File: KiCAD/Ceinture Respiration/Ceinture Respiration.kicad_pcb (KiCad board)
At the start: 4 copper layers, 45 x 82.8 mm, 39 parts, among them J1 Conn_01x10_Pin, J10 BUZZER, J11 Conn_01x02, J2 Conn_01x10_Socket, J3 Conn_01x06_Pin, J4 Conn_01x06_Pin, J5 Conn_01x06_Pin, J6 DIN-8, J7 DIN-8, J8 Oled, J9 MEM2061-01-188-00-A_REVA, M1 Motor_DC, Q1 MMBT3904, Q2 AP10N04S, SW1 SW_Push, SW2 SW_Push, SW3 SW_Push, SW4 SW_Push, U1 DRV2605LDGS

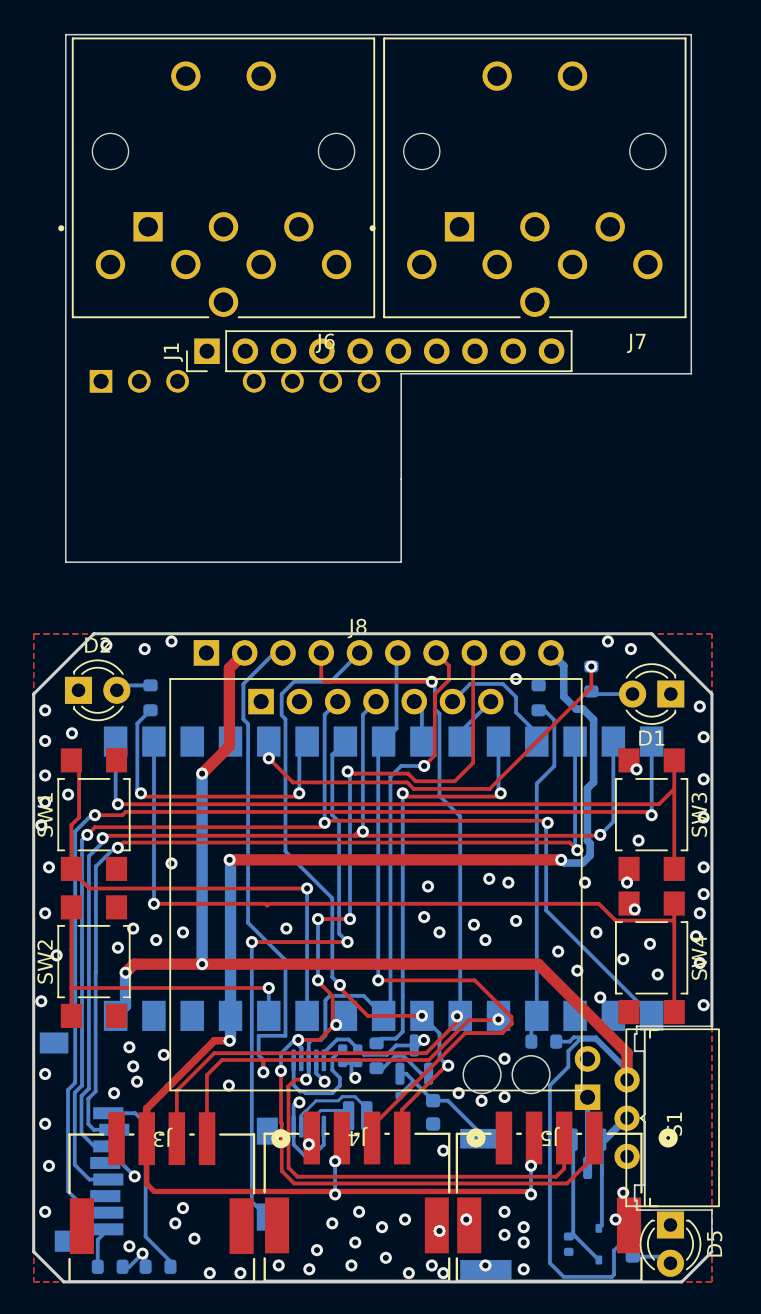
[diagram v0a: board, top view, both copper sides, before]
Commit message: sch 99% pcb 99%
Reste à préparer les commandes
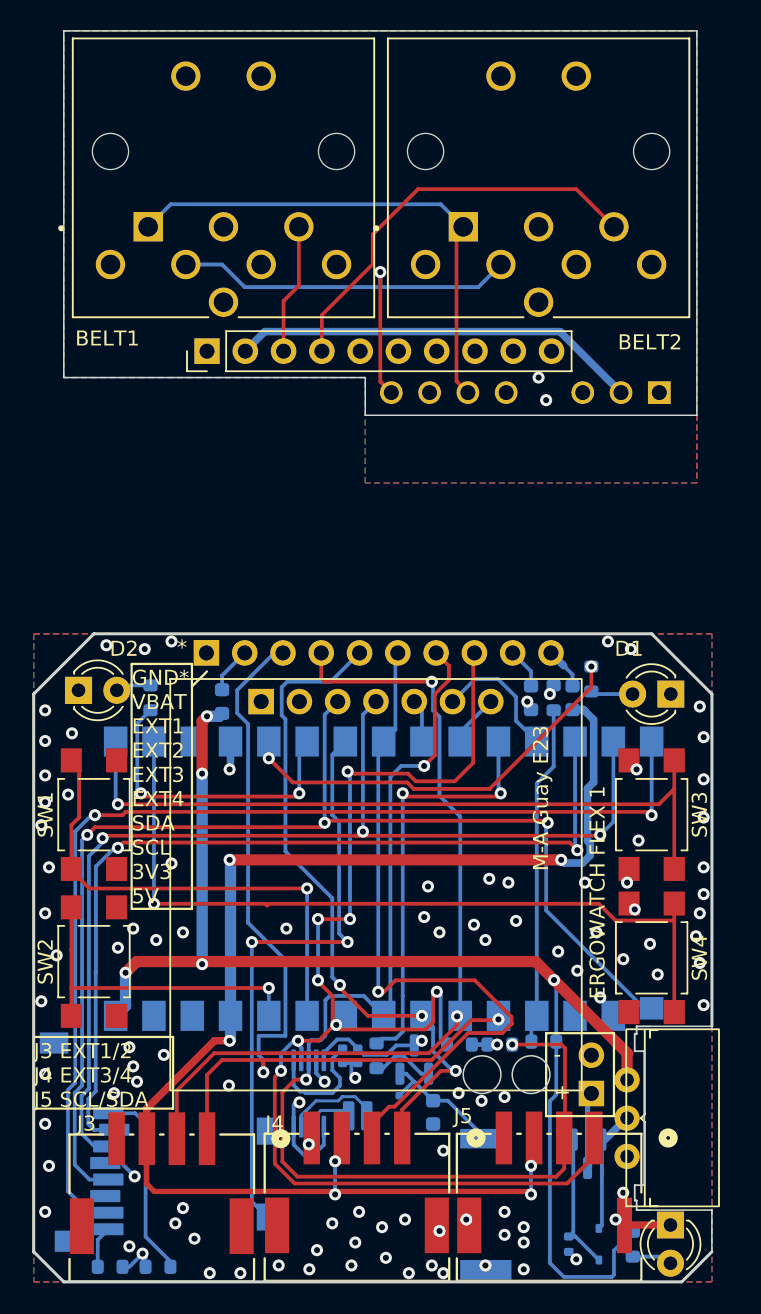
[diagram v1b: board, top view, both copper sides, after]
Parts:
- added F1: 500mA, Fuse:Fuse_0603_1608Metric, B.Cu at (164.0, 117.0)
- added F2: 500mA, Fuse:Fuse_0603_1608Metric, B.Cu at (166.8, 117.0)
- added F3: 500mA, Fuse:Fuse_0603_1608Metric, B.Cu at (143.5, 117.2)
- added R10: 10K, Resistor_SMD:R_0603_1608Metric, B.Cu at (159.2, 140.0)
- added R11: 10K, Resistor_SMD:R_0603_1608Metric, B.Cu at (161.9, 140.0)
- moved PS1 19.6 mm to (163.6, 98.1), turned to 180 degrees
- moved R2 1.00 mm to (165.5, 117.0)
- moved J11 0.35 mm to (168.0, 143.2)
- moved J7 0.25 mm to (164.5, 80.8)
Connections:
- J2 pad 10: +5V -> Net-(J2-Pin_10)
- J2 pad 2: /BATTERIE 9V/VBAT -> Net-(J2-Pin_2)
- J2 pad 9: +3.3V -> Net-(J2-Pin_9)
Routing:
- net +5VA: track 0.00 -> 33.6 mm
- net -5VA: track 0.00 -> 31.4 mm, vias 0 -> 1
- net /SHIELD_RESPIRATION/Belt_2: track 0.00 -> 27.4 mm
- net /SHIELD_RESPIRATION/VBAT_EXP: track 0.00 -> 27.1 mm
- net +3.3V: track 21.8 -> 41.9 mm, vias 5 -> 7
- net /SCL: track 72.8 -> 85.7 mm, vias 7 -> 8
- net /BATTERIE 9V/VBAT: track 97.4 -> 86.9 mm, vias 3 -> 5
- net /SDA: track 65.4 -> 75.3 mm, vias 2 -> 3
- net /SHIELD_RESPIRATION/Belt_1: track 0.00 -> 8.67 mm
- net GND: track 5.72 -> 10.9 mm, vias 99 -> 100
- net Net-(J2-Pin_10): track 0.00 -> 3.99 mm
- net +5V: track 97.4 -> 93.4 mm
- net Net-(J2-Pin_2): track 0.00 -> 3.06 mm
- net Net-(J2-Pin_9): track 0.00 -> 2.70 mm
- net /MCU/EXT3: track 43.9 -> 45.1 mm
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- added copper zone on B.Cu, net GND_EXP
- added copper zone on F.Cu, net GND_EXP
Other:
- board size 45 x 82.8 mm -> 45 x 83 mm
- board text added: "*"
- board text added: "+"
- board text added: "-"
- board text added: "5-12V"
- board text added: "BELT1"
- board text added: "BELT2"
- board text added: "ERGOWATCH FLEX 1"
- board text added: "GND* VBAT EXT1 EXT2 EXT3 EXT4 SDA SCL 3V3 5V"
- board text added: "IngRéadapt - ULaval - CIRRIS"
- board text added: "IngRéadapt-ULaval-CIRRIS"
- board text added: "J3 EXT1/2 J4 EXT3/4 J5 SCL/SDA"
- board text added: "M-A Guay E23"
- board text added: "Module externe pour ceintures de respiration"
